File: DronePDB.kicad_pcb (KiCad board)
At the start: 2 copper layers, 50 x 50 mm, 23 parts, among them J1 OUT, J2 OUT, J3 OUT, J4 OUT, J5 OUT, J6 OUT, J7 OUT, U1 12V Reg 1, U2 12V Reg 2, U3 9V Reg 1, U4 9V Reg 2, U5 5V Reg 1, U6 5V Reg 2, U7 5V Reg 3

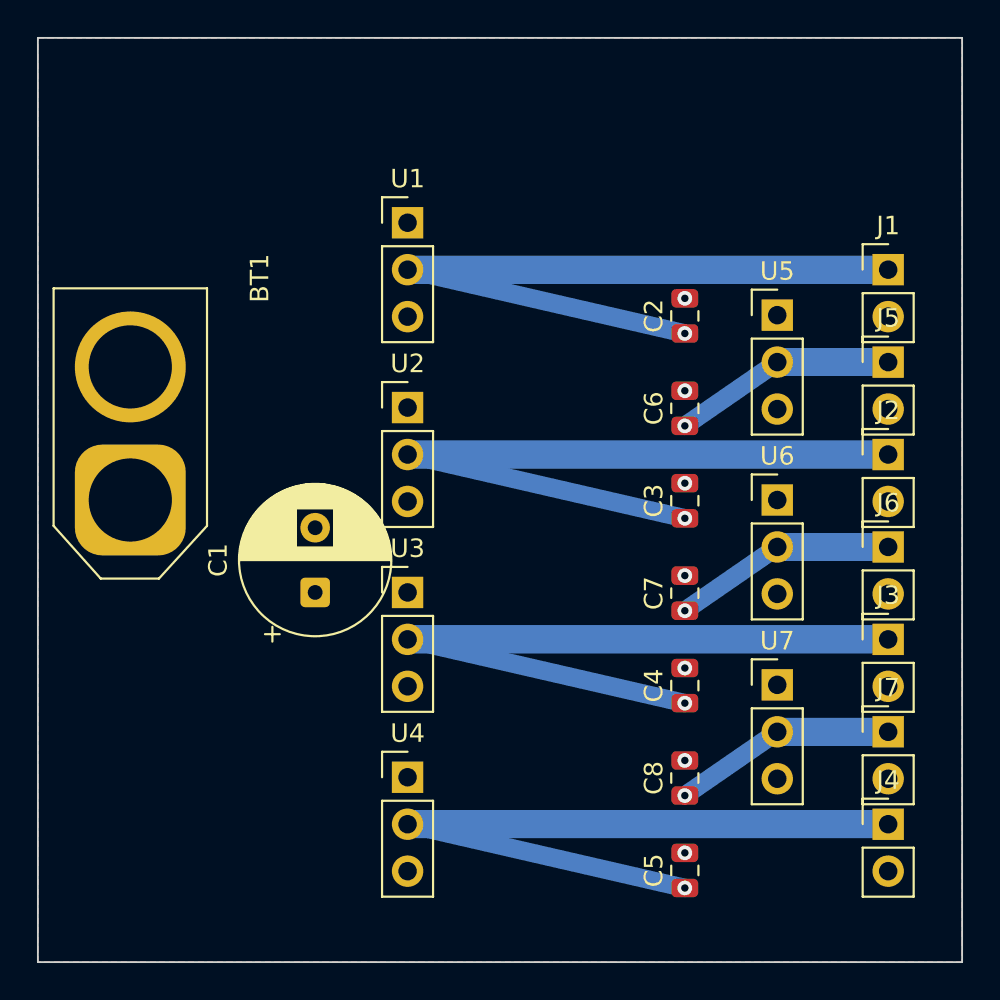
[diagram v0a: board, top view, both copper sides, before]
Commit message: update
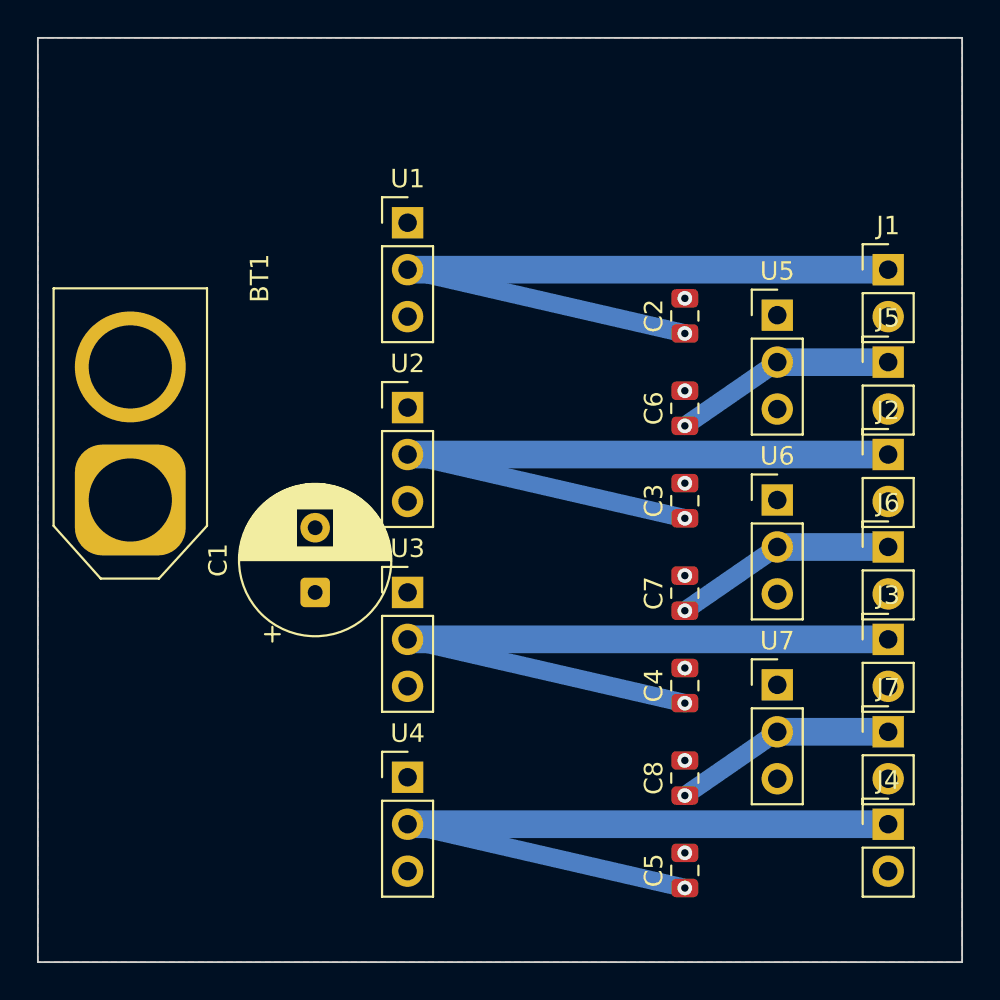
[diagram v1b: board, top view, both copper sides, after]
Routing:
- net VOUT_9V_2: track 67.4 -> 41.4 mm
- net VOUT_9V_1: track 67.4 -> 41.4 mm
- net VOUT_12V_2: track 67.4 -> 41.4 mm
- net VOUT_12V_1: track 67.4 -> 41.4 mm
- net VOUT_5V_3: track 18.1 -> 12.1 mm
- net VOUT_5V_2: track 18.1 -> 12.1 mm
- net VOUT_5V_1: track 18.1 -> 12.1 mm
- net GND: vias 23 -> 7
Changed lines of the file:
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@@
-	)
-	(segment
-		(start 40 37.54)
-		(end 46 37.54)
-		(width 1.5)
-		(layer "B.Cu")
-		(net 1)
 	)
 	(segment
@@
 	)
 	(segment
-		(start 40 27.54)
-		(end 46 27.54)
-		(width 1.5)
+		(start 35 30.99)
+		(end 40 27.54)
+		(width 1)
 		(layer "B.Cu")
 		(net 2)
@@
 		(end 46 27.54)
 		(width 1.5)
-		(layer "B.Cu")
-		(net 2)
-	)
-	(segment
-		(start 35 30.99)
-		(end 40 27.54)
-		(width 1)
 		(layer "B.Cu")
 		(net 2)
@@
 		(net 3)
 	)
-	(segment
-		(start 20 32.54)
-		(end 46 32.54)
-		(width 1.5)
-		(layer "B.Cu")
-		(net 3)
-	)
 	(via
 		(at 35 15.99)
@@
 		(drill 0.4)
 		(layers "F.Cu" "B.Cu")
-		(net 4)
-	)
-	(segment
-		(start 20 12.54)
-		(end 46 12.54)
-		(width 1.5)
-		(layer "B.Cu")
 		(net 4)
 	)
@@
 	)
 	(segment
-		(start 20 42.54)
-		(end 46 42.54)
-		(width 1.5)
-		(layer "B.Cu")
-		(net 5)
-	)
-	(segment
 		(start 35 45.99)
 		(end 20 42.54)
@@
 		(drill 0.4)
 		(layers "F.Cu" "B.Cu")
-		(net 6)
-	)
-	(segment
-		(start 20 22.54)
-		(end 46 22.54)
-		(width 1.5)
-		(layer "B.Cu")
 		(net 6)
 	)
@@
 		(net 7)
 	)
-	(segment
-		(start 40 17.54)
-		(end 46 17.54)
-		(width 1.5)
-		(layer "B.Cu")
-		(net 7)
-	)
 	(via
-		(at 35 14.09)
+		(at 35 29.09)
 		(size 0.8)
 		(drill 0.4)
@@
 	)
 	(via
-		(at 46 30.08)
-		(size 0.8)
-		(drill 0.4)
-		(layers "F.Cu" "B.Cu")
-		(net 8)
-	)
-	(via
-		(at 40 40.08)
-		(size 0.8)
-		(drill 0.4)
-		(layers "F.Cu" "B.Cu")
-		(net 8)
-	)
-	(via
-		(at 20 25.08)
-		(size 0.8)
-		(drill 0.4)
-		(layers "F.Cu" "B.Cu")
-		(net 8)
-	)
-	(via
-		(at 46 40.08)
+		(at 35 34.09)
 		(size 0.8)
 		(drill 0.4)
@@
 	)
 	(via
-		(at 15 26.5)
+		(at 35 44.09)
 		(size 0.8)
 		(drill 0.4)
@@
 	)
 	(via
-		(at 20 35.08)
-		(size 0.8)
-		(drill 0.4)
-		(layers "F.Cu" "B.Cu")
-		(net 8)
-	)
-	(via
-		(at 46 15.08)
-		(size 0.8)
-		(drill 0.4)
-		(layers "F.Cu" "B.Cu")
-		(net 8)
-	)
-	(via
-		(at 46 20.08)
-		(size 0.8)
-		(drill 0.4)
-		(layers "F.Cu" "B.Cu")
-		(net 8)
-	)
-	(via
-		(at 46 25.08)
-		(size 0.8)
-		(drill 0.4)
-		(layers "F.Cu" "B.Cu")
-		(net 8)
-	)
-	(via
-		(at 35 44.09)
+		(at 35 14.09)
 		(size 0.8)
 		(drill 0.4)
@@
 	)
 	(via
-		(at 40 20.08)
-		(size 0.8)
-		(drill 0.4)
-		(layers "F.Cu" "B.Cu")
-		(net 8)
-	)
-	(via
-		(at 5 17.8)
-		(size 0.8)
-		(drill 0.4)
-		(layers "F.Cu" "B.Cu")
-		(net 8)
-	)
-	(via
-		(at 20 15.08)
-		(size 0.8)
-		(drill 0.4)
-		(layers "F.Cu" "B.Cu")
-		(net 8)
-	)
-	(via
-		(at 46 45.08)
-		(size 0.8)
-		(drill 0.4)
-		(layers "F.Cu" "B.Cu")
-		(net 8)
-	)
-	(via
-		(at 35 34.09)
-		(size 0.8)
-		(drill 0.4)
-		(layers "F.Cu" "B.Cu")
-		(net 8)
-	)
-	(via
 		(at 35 39.09)
 		(size 0.8)
 		(drill 0.4)
-		(layers "F.Cu" "B.Cu")
-		(net 8)
-	)
-	(via
-		(at 40 30.08)
-		(size 0.8)
-		(drill 0.4)
-		(layers "F.Cu" "B.Cu")
-		(net 8)
-	)
-	(via
-		(at 46 35.08)
-		(size 0.8)
-		(drill 0.4)
-		(layers "F.Cu" "B.Cu")
-		(net 8)
-	)
-	(via
-		(at 35 29.09)
-		(size 0.8)
-		(drill 0.4)
-		(layers "F.Cu" "B.Cu")
-		(net 8)
-	)
-	(via
-		(at 20 45.08)
-		(size 0.8)
-		(drill 0.4)
